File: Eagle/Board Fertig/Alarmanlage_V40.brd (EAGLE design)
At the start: 102.2 x 84.1 mm, 85 parts, among them IC02 3.3V, IC05 5V, IC1 MC9S08AW60, Q1 4M9152, Q2 P5N50D

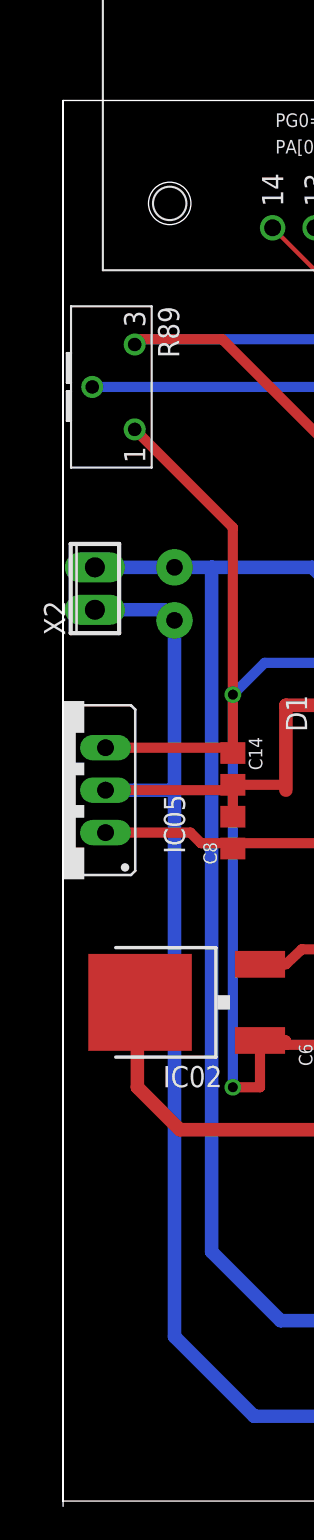
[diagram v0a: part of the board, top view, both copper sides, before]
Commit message: add Board
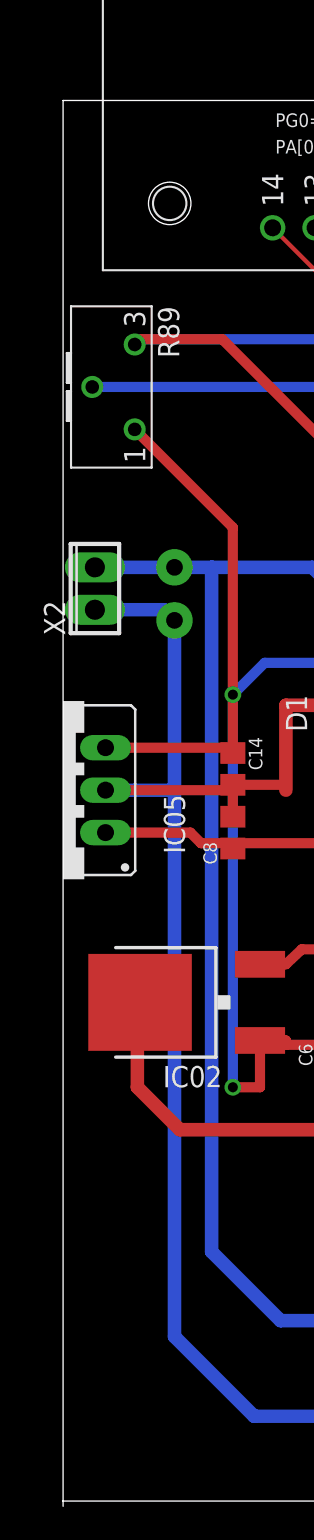
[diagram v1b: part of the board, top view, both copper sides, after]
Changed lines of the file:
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@@
 <setting verticaltext="up"/>
 </settings>
-<grid distance="0.05" unitdist="inch" unit="mil" style="lines" multiple="1" display="no" altdistance="0.025" altunitdist="inch" altunit="inch"/>
+<grid distance="12.5" unitdist="mil" unit="mil" style="dots" multiple="1" display="yes" altdistance="0.025" altunitdist="inch" altunit="inch"/>
 <layers>
 <layer number="1" name="Top" color="4" fill="1" visible="yes" active="yes"/>
@@
 Schuljahr 2013/14</text>
 <text x="2.8575" y="10.16" size="3.81" layer="27">Alarmanlage</text>
-<wire x1="0.635" y1="84.1375" x2="0.635" y2="0" width="0.0254" layer="46"/>
+<wire x1="0.635" y1="0.3175" x2="0.635" y2="0" width="0.0254" layer="46"/>
 </plain>
 <attributes>
